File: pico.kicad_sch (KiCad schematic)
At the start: 7 parts, among them J12 I2C, Q4 DMG2305UX, U14 Pico

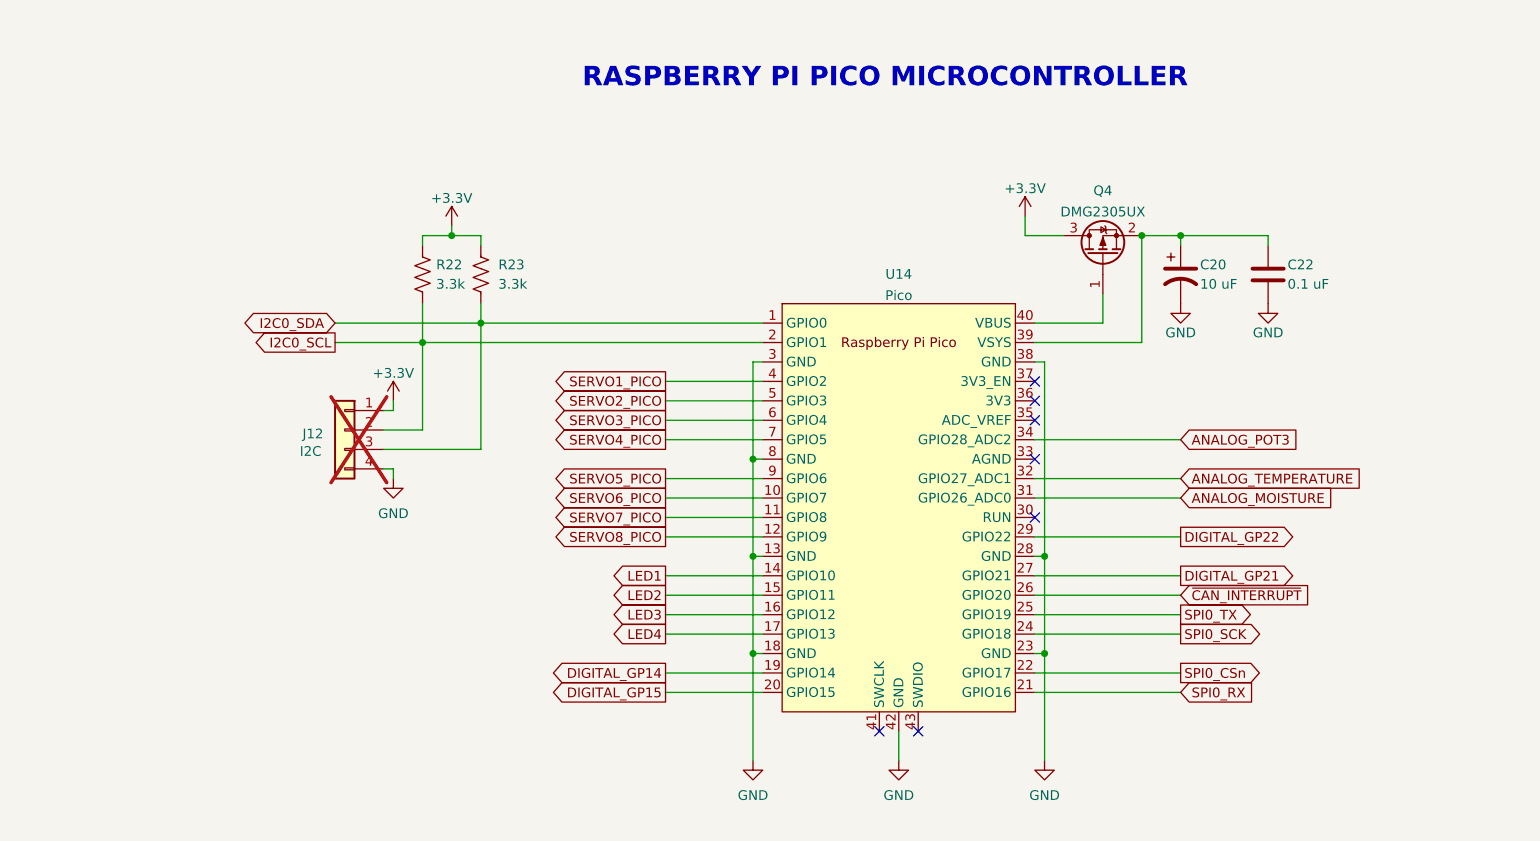
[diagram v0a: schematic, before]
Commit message: major rework again after the meeting
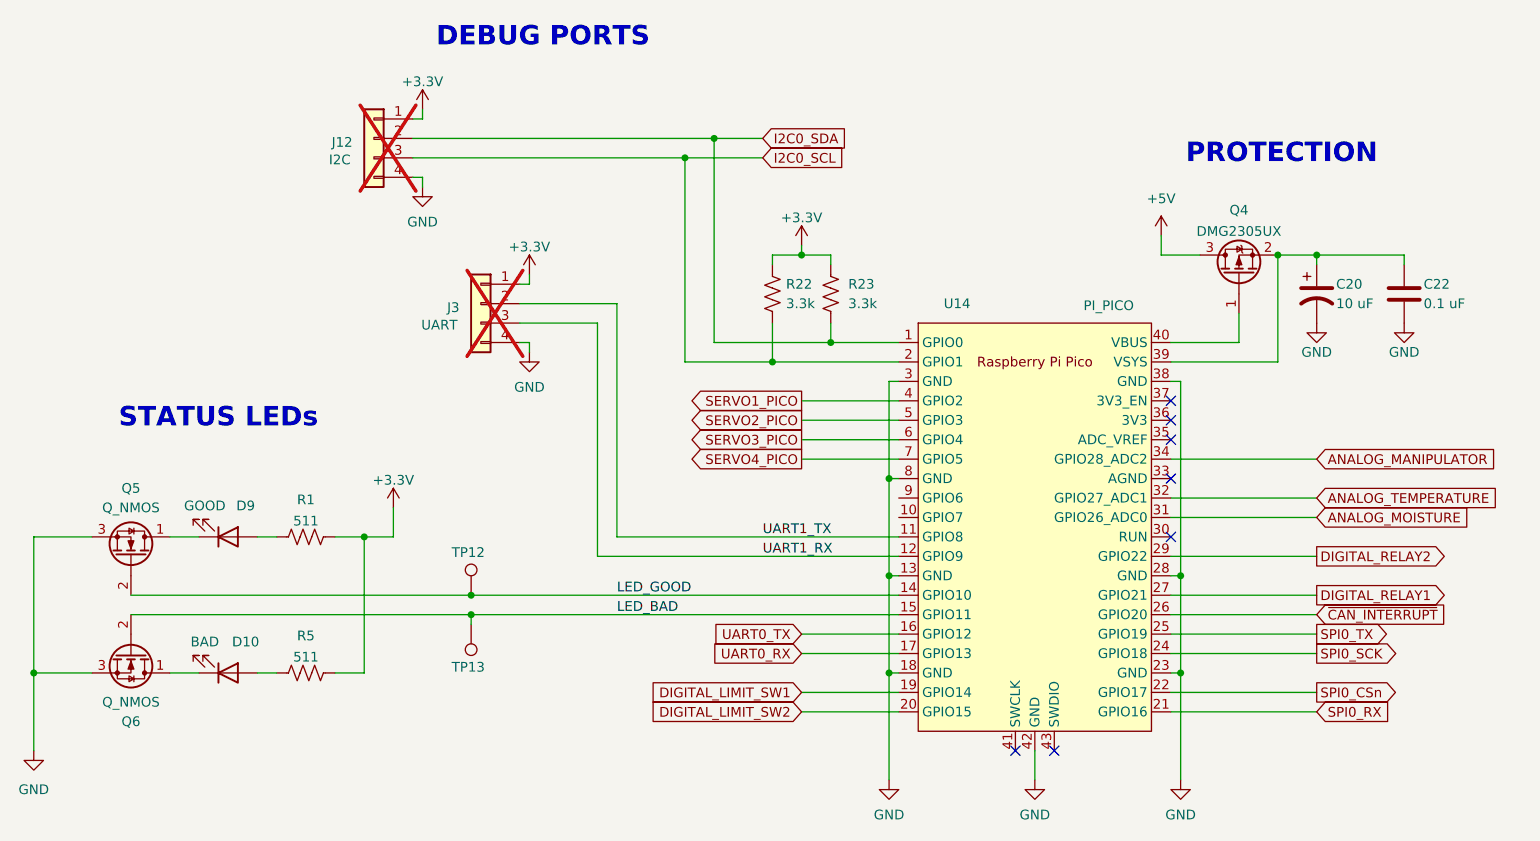
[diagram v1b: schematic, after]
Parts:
- added D10: BAD, LED_SMD:LED_0805_2012Metric_Pad1.15x1.40mm_HandSolder, symbol Device:LED
- added D9: GOOD, LED_SMD:LED_0805_2012Metric_Pad1.15x1.40mm_HandSolder, symbol Device:LED
- added J3: UART, Connector_Molex:Molex_PicoBlade_53047-0410_1x04_P1.25mm_Vertical, symbol Connector_Generic:Conn_01x04
- added Q5, Q6: Q_NMOS, Package_TO_SOT_SMD:TSOT-23, symbol Transistor_FET:Q_NMOS_DGS
- added R1, R5: 511, Resistor_SMD:R_0805_2012Metric_Pad1.20x1.40mm_HandSolder, symbol Device:R_US
- added TP12: LED1, TestPoint:TestPoint_Pad_D1.0mm, symbol Connector:TestPoint
- added TP13: LED2, TestPoint:TestPoint_Pad_D1.0mm, symbol Connector:TestPoint
- C20: footprint Payload_PCB_v3.1:UCM1H220MCL1GS -> Capacitor_SMD:C_Elec_4x5.4
- U14: value Pico -> PI_PICO
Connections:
- net +3.3V: now also J3.1 (Pin_1), R1.2, R5.2; no longer Q4.3 (D)
- net GND: now also J3.4 (Pin_4), Q5.3 (S), Q6.3 (S)
- net I2C0_SCL: now also J12.3 (Pin_3); no longer J12.2 (Pin_2)
- net I2C0_SDA: now also J12.2 (Pin_2); no longer J12.3 (Pin_3)
- net ANALOG_POT3 renamed ANALOG_MANIPULATOR
- net DIGITAL_GP14 renamed DIGITAL_LIMIT_SW1
- net DIGITAL_GP15 renamed DIGITAL_LIMIT_SW2
- net DIGITAL_GP21 renamed DIGITAL_RELAY1
- net DIGITAL_GP22 renamed DIGITAL_RELAY2
- net LED1 renamed LED_GOOD
- net LED_GOOD: now also Q5.2 (G), TP12.1
- net LED2 renamed LED_BAD
- net LED_BAD: now also Q6.2 (G), TP13.1
- net LED3 renamed UART0_TX
- net LED4 renamed UART0_RX
- net SERVO5_PICO: no longer names the net of U14.9 (GPIO6)
- net SERVO6_PICO: no longer names the net of U14.10 (GPIO7)
- net SERVO7_PICO renamed UART1_TX
- net UART1_TX: now also J3.2 (Pin_2)
- net SERVO8_PICO renamed UART1_RX
- net UART1_RX: now also J3.3 (Pin_3)
- new net: D9.1 (K), Q5.1 (D)
- new net: D9.2 (A), R1.1
- new net: D10.1 (K), Q6.1 (D)
- new net: D10.2 (A), R5.1
- new net +5V: Q4.3 (D)
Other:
- note added: "DEBUG PORTS"
- note added: "PROTECTION"
- note added: "STATUS LEDs"
- note removed: "RASPBERRY PI PICO MICROCONTROLLER"
- moved on the sheet: C20, C22, J12, Q4, R22, R23, U14
